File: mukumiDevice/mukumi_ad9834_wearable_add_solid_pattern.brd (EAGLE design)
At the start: 49.2 x 41.7 mm, 136 parts, among them IC1 AD835, IC10 NJM2884, IC11 AD9834, IC12 AD9834, IC13 SIT8002B, IC2 AD835, IC3 AD835, IC4 TL072D, IC5 NJM074V, IC6 NJM074V, IC7 NJM074V, IC8 NJM074V, IC9 NJM2884

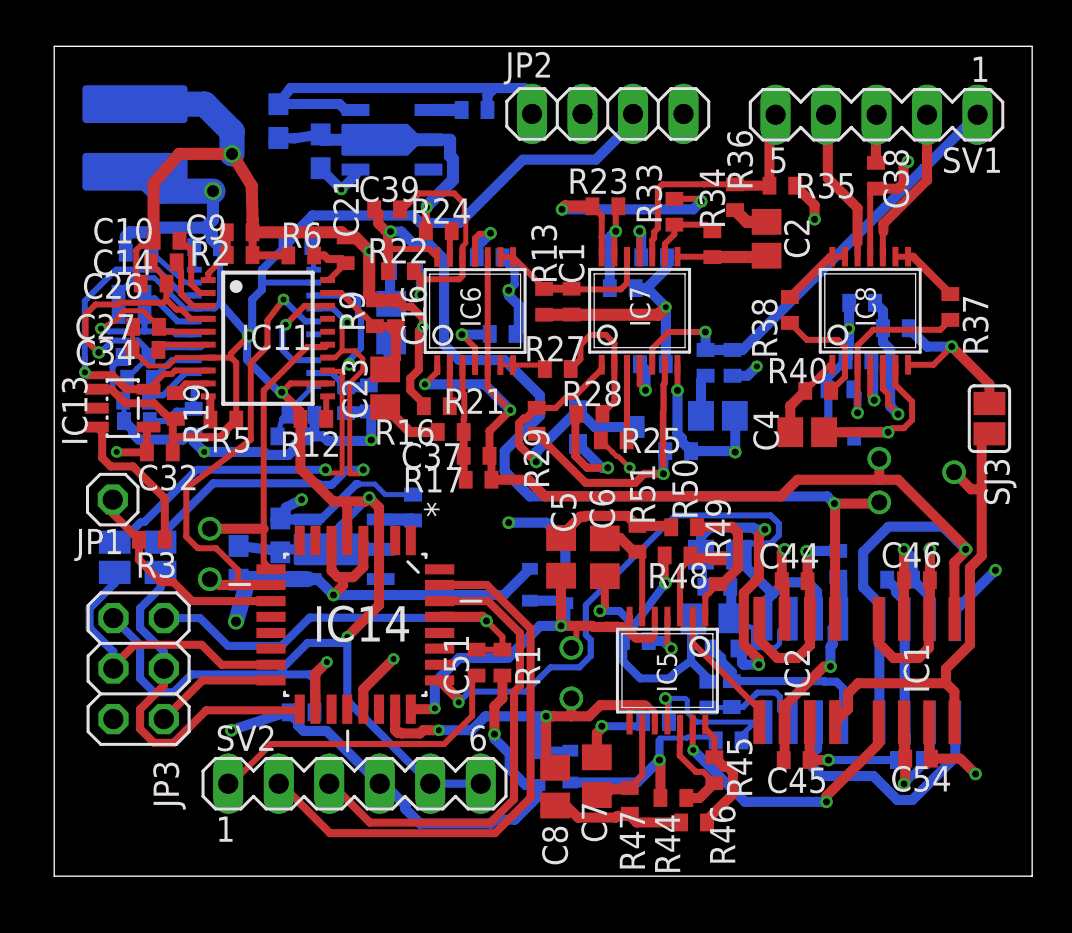
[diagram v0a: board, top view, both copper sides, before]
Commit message: brd,schの修正,utility追加
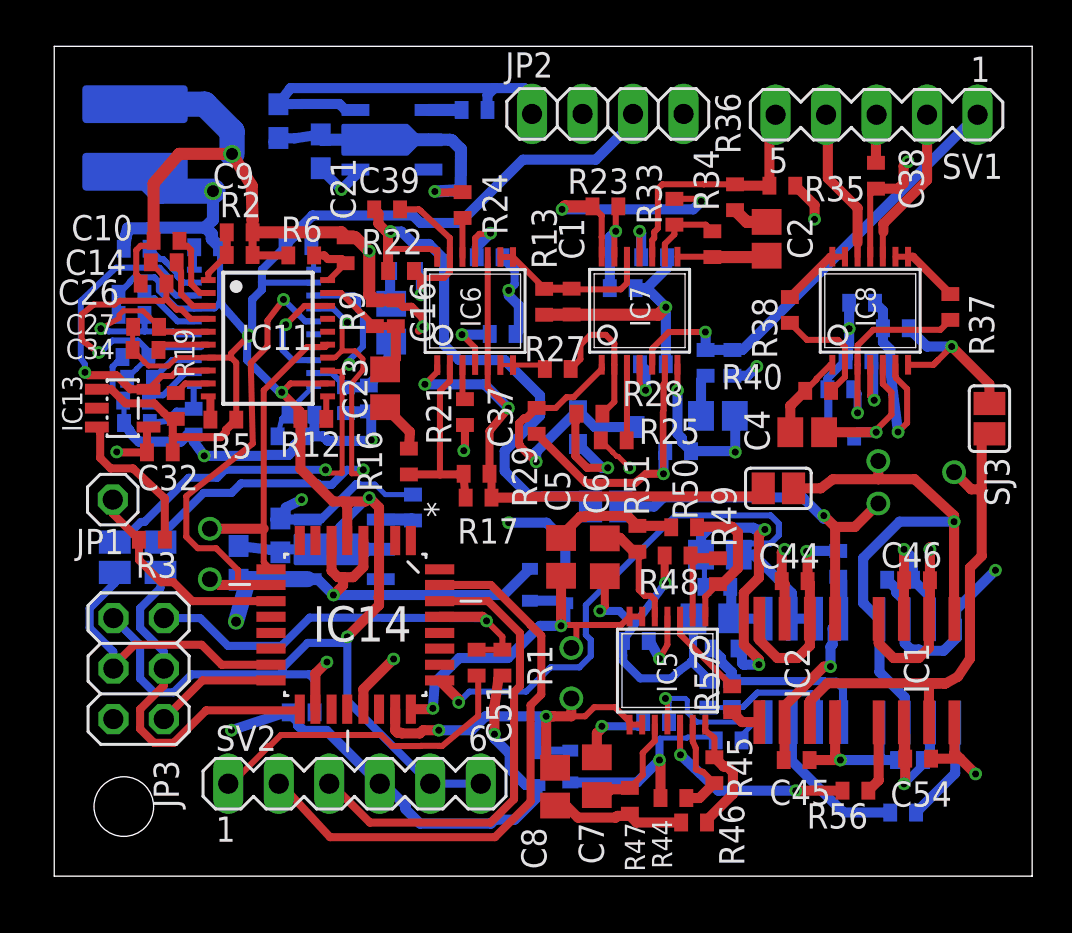
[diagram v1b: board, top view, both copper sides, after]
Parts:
- added R56, R57, R58: 560a, rcl:R0402
- added SJ4, SJ5: (no value), jumper:SJ
- moved R16 2.57 mm to (17.8, 20.9), turned to 90 degrees
- moved R24 1.78 mm to (20.5, 33.8), turned to 90 degrees
- moved R21 1.45 mm to (20.7, 23.3), turned to 270 degrees
- moved C37 0.90 mm to (21.2, 20.2)
- moved R17 0.90 mm to (21.3, 19.0)
- moved R4 0.22 mm to (4.15, 31.6)
- moved R18 0.10 mm to (4.16, 22.8)
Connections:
- removed net N$39: IC6.13, R24.1
- removed net N$45: IC2.5, IC5.2
- removed net N$68: IC3.5, IC4.2
- new net COS_: IC2.1, SJ5.2
- new net N$15: IC6.12, R24.1
- new net N$16: IC4.3, R58.2
- new net N$18: IC2.5, R57.1
- new net N$21: IC5.3, R57.2
- new net N$23: IC1.5, R56.1
- new net N$24: IC5.12, R56.2
- new net SIN_: IC1.1, IC3.1, IC3.7, SJ4.2
- net AGND: now also IC1.8, IC2.8, IC3.8; no longer IC1.7, IC2.7, IC3.7
- net COS: now also SJ5.1; no longer IC2.1
- net N$1: now also IC6.3; no longer IC6.2
- net N$17: now also IC5.13; no longer IC5.12
- net N$19: now also IC4.5; no longer IC4.6
- net N$2: now also IC5.5; no longer IC5.6
- net N$3: now also IC5.10; no longer IC5.9
- net N$43: now also IC5.2; no longer IC5.3
- net N$5: now also IC3.5, R58.1; no longer IC1.5, IC5.13
- net N$55: now also IC8.5; no longer IC8.6
- net N$58: now also IC8.6; no longer IC8.5
- net N$70: now also IC4.2; no longer IC4.3
- net N$78: now also IC6.2; no longer IC6.3
- net N$91: now also IC6.13; no longer IC6.12
- net SIG*COS: now also IC5.6; no longer IC5.5
- net SIG*SIN: now also IC5.9; no longer IC5.10
- net SIG_: now also IC1.7, IC2.7; no longer IC1.8, IC2.8
- net SIN: now also SJ4.1; no longer IC1.1, IC3.1, IC3.8
- net SIN*SIN: now also IC4.6; no longer IC4.5
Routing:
- net SIN: track 64.5 -> 32.7 mm, vias 4 -> 2
- net SIN_: track 0.00 -> 30.0 mm, vias 0 -> 2
- net COS: track 49.8 -> 29.9 mm, vias 3 -> 1
- net COS_: track 0.00 -> 19.1 mm, vias 0 -> 2
- net N$68: track 12.8 -> 0.00 mm
- net AGND: track 357.1 -> 367.9 mm, vias 24 -> 25
- net N$24: track 0.00 -> 10.4 mm, vias 0 -> 2
- net N$5: track 14.2 -> 5.34 mm, vias 2 -> 0
- net N$16: track 0.00 -> 7.98 mm
- net SIG*COS: track 28.7 -> 21.4 mm
- net N$45: track 6.70 -> 0.00 mm
- net N$21: track 0.00 -> 4.59 mm
- net N$78: track 5.86 -> 9.75 mm
- net N$23: track 0.00 -> 3.65 mm
- net N$91: track 12.6 -> 9.39 mm
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
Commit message: 負電圧の信号を取るため、atmega328のPWM(analogWrite)とRCローパスを用いてVCC/2を生成し、それを抵抗(1.8kのやつ）で加算してからAD変換ポートにつなぐ
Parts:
- R20: value 1k -> 680
- R23: value 1k -> 360
- R28: value 2k -> 1k
- R45: value 100k -> 11k
- R49: value 47k -> 11k
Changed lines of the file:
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@@
 <attribute name="VALUE" x="34.6538" y="20.6098" size="1.27" layer="28" rot="MR0"/>
 </element>
-<element name="R20" library="rcl" library_urn="urn:adsk.eagle:library:334" package="R0402" value="1k" x="28.5958" y="29.5778" smashed="yes" rot="MR0">
+<element name="R20" library="rcl" library_urn="urn:adsk.eagle:library:334" package="R0402" value="680" x="28.5958" y="29.5778" smashed="yes" rot="MR0">
 <attribute name="NAME" x="29.5356" y="27.4188" size="1.27" layer="26" rot="MR0"/>
 <attribute name="VALUE" x="29.2308" y="27.6728" size="1.27" layer="28" rot="MR0"/>
 </element>
-<element name="R23" library="rcl" library_urn="urn:adsk.eagle:library:334" package="R0402" value="1k" x="27.7238" y="33.6898" smashed="yes">
+<element name="R23" library="rcl" library_urn="urn:adsk.eagle:library:334" package="R0402" value="360" x="27.7238" y="33.6898" smashed="yes">
 <attribute name="NAME" x="25.8188" y="34.3248" size="1.27" layer="25"/>
 <attribute name="VALUE" x="27.0888" y="31.7848" size="1.27" layer="27"/>
@@
 <attribute name="VALUE" x="25.9628" y="27.4168" size="1.27" layer="27" rot="R180"/>
 </element>
-<element name="R28" library="rcl" library_urn="urn:adsk.eagle:library:334" package="R0402" value="2k" x="26.9238" y="23.2598" smashed="yes">
+<element name="R28" library="rcl" library_urn="urn:adsk.eagle:library:334" package="R0402" value="1k" x="26.9238" y="23.2598" smashed="yes">
 <attribute name="NAME" x="28.5748" y="23.6408" size="1.27" layer="25"/>
 <attribute name="VALUE" x="26.2888" y="21.3548" size="1.27" layer="27"/>
@@
 <attribute name="VALUE" x="41.6988" y="29.4648" size="1.27" layer="28" rot="MR180"/>
 </element>
-<element name="R45" library="rcl" package="R0402" value="100k" x="33.2038" y="5.3298" smashed="yes" rot="R90">
+<element name="R45" library="rcl" package="R0402" value="11k" x="33.2038" y="5.3298" smashed="yes" rot="R90">
 <attribute name="NAME" x="35.1088" y="3.9328" size="1.27" layer="25" rot="R90"/>
 <attribute name="VALUE" x="35.1088" y="4.6948" size="1.27" layer="27" rot="R90"/>
 </element>
-<element name="R49" library="rcl" package="R0402" value="47k" x="33.3838" y="15.3398" smashed="yes" rot="R270">
+<element name="R49" library="rcl" package="R0402" value="11k" x="33.3838" y="15.3398" smashed="yes" rot="R270">
 <attribute name="NAME" x="33.0536" y="19.6324" size="1.27" layer="25" rot="R270"/>
 <attribute name="VALUE" x="31.4788" y="15.9748" size="1.27" layer="27" rot="R270"/>
